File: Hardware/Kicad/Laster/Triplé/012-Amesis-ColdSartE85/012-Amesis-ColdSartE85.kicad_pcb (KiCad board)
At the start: 2 copper layers, 52.1 x 54.9 mm, 24 parts, among them J1 Screw_Terminal_01x02, J2 Conn_01x05_Female, J3 Conn_01x03_Female

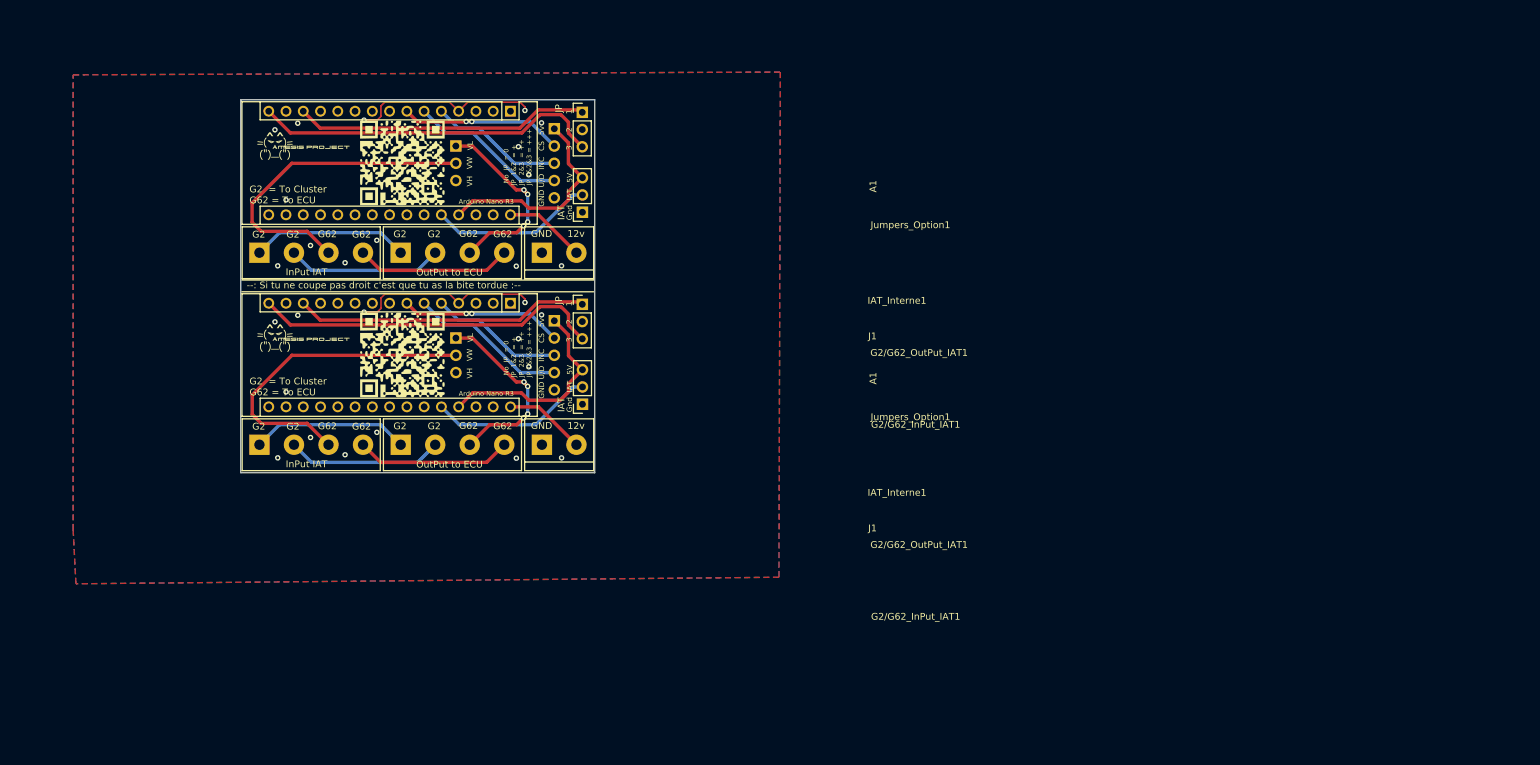
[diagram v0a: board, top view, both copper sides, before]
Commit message: maj
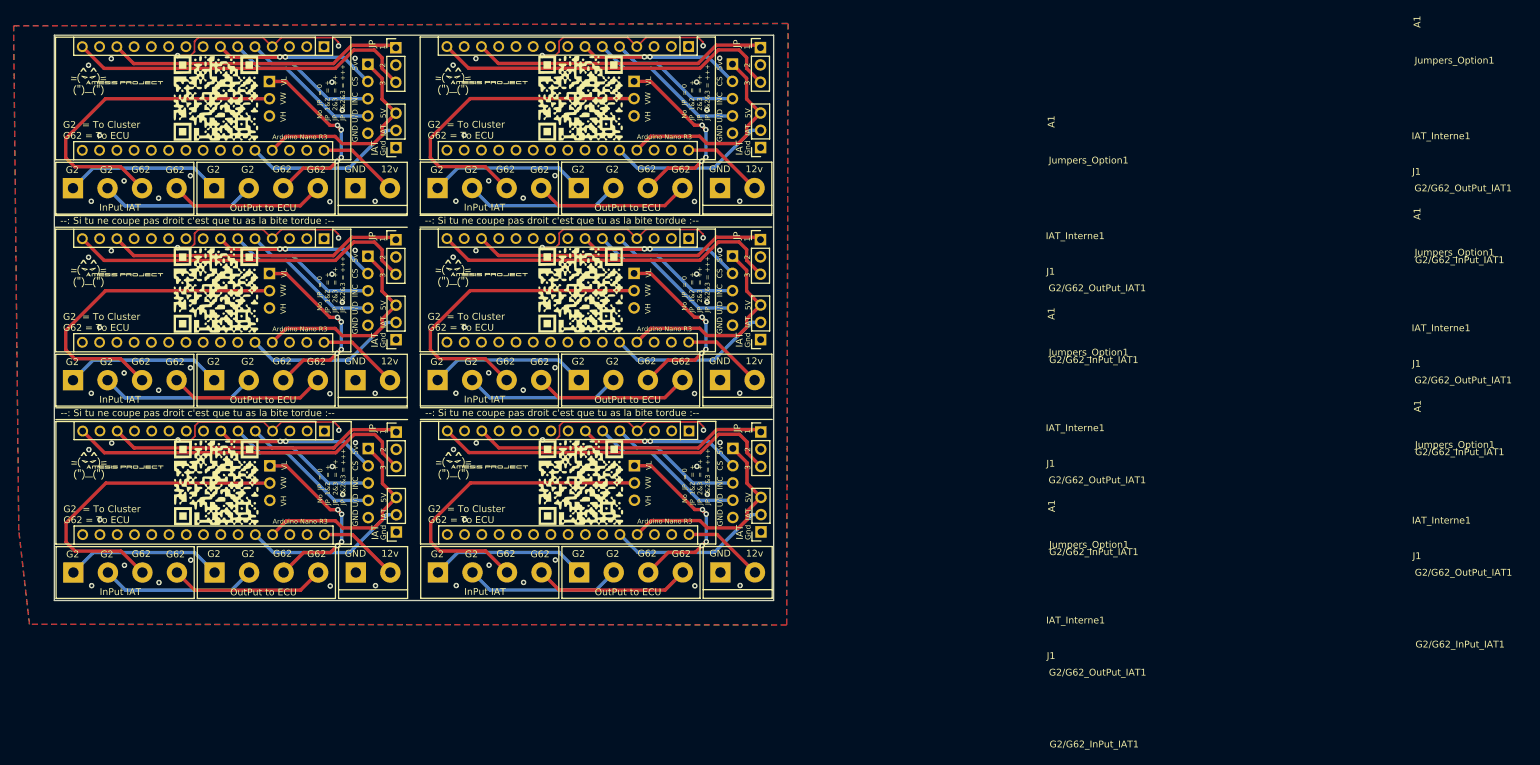
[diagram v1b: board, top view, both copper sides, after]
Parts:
- added  : LOGO, AP_Amesis Logo:AmesisProject Logo 15mm, F.Cu at (99.0, 51.5)
- added  : LOGO, AP_Amesis Logo:AmesisProject Logo 15mm, F.Cu at (99.1, 79.8)
- added  : LOGO, AP_Amesis Logo:AmesisProject Logo 30mm, B.Cu at (105.5, 51.7)
- added  : LOGO, AP_Amesis Logo:10x10 KiCad QR Code La Boutique Amesis Project, B.Cu at (128.8, 24.2)
- added  : LOGO, AP_Amesis Logo:AmesisProject Logo 30mm, B.Cu at (105.5, 80.0)
- added  : LOGO, AP_Amesis Logo:AmesisProject Logo 30mm, B.Cu at (105.5, 23.5)
- added  : LOGO, AP_Amesis Logo:10x10 KiCad QR Code La Boutique Amesis Project, B.Cu at (182.5, 80.7)
- added  : LOGO, AP_Amesis Logo:10x10 KiCad QR Code La Boutique Amesis Project, B.Cu at (128.9, 80.8)
- added  : LOGO, AP_Amesis Logo:15x15 KiCad QR Code La Boutique Amesis Project, F.Cu at (167.4, 81.5)
- added  : LOGO, AP_Amesis Logo:10x10 KiCad QR Code La Boutique Amesis Project, B.Cu at (128.8, 52.5)
- added  : LOGO, AP_Amesis Logo:AmesisProject Logo 30mm, B.Cu at (159.2, 80.0)
- added  : LOGO, AP_Amesis Logo:15x15 KiCad QR Code La Boutique Amesis Project, F.Cu at (113.8, 81.5)
- added  : LOGO, AP_Amesis Logo:15x15 KiCad QR Code La Boutique Amesis Project, F.Cu at (113.7, 24.9)
- added  : LOGO, AP_Amesis Logo:AmesisProject Logo 15mm, F.Cu at (99.0, 23.3)
- added  : LOGO, AP_Amesis Logo:AmesisProject Logo 15mm, F.Cu at (152.7, 79.8)
- added  : LOGO, AP_Amesis Logo:15x15 KiCad QR Code La Boutique Amesis Project, F.Cu at (113.7, 53.2)
- added A1: Arduino_Nano_v3.x, Module:Arduino_Nano, F.Cu at (129.6, 45.8)
- added A1: Arduino_Nano_v3.x, Module:Arduino_Nano, F.Cu at (183.3, 74.1)
- added A1: Arduino_Nano_v3.x, Module:Arduino_Nano, F.Cu at (129.7, 74.1)
- added A1: Arduino_Nano_v3.x, Module:Arduino_Nano, F.Cu at (129.6, 17.6)
- added G2/G62_InPut_IAT1: Conn_01x04_Male, TerminalBlock:TerminalBlock_bornier-4_P5.08mm, F.Cu at (146.4, 94.9)
- added G2/G62_InPut_IAT1: Conn_01x04_Male, TerminalBlock:TerminalBlock_bornier-4_P5.08mm, F.Cu at (92.7, 38.4)
- added G2/G62_InPut_IAT1: Conn_01x04_Male, TerminalBlock:TerminalBlock_bornier-4_P5.08mm, F.Cu at (92.8, 95.0)
- added G2/G62_InPut_IAT1: Conn_01x04_Male, TerminalBlock:TerminalBlock_bornier-4_P5.08mm, F.Cu at (92.7, 66.7)
- added G2/G62_OutPut_IAT1: Conn_01x04_Male, TerminalBlock:TerminalBlock_bornier-4_P5.08mm, F.Cu at (113.5, 66.7)
- added G2/G62_OutPut_IAT1: Conn_01x04_Male, TerminalBlock:TerminalBlock_bornier-4_P5.08mm, F.Cu at (113.5, 38.4)
- added G2/G62_OutPut_IAT1: Conn_01x04_Male, TerminalBlock:TerminalBlock_bornier-4_P5.08mm, F.Cu at (167.2, 94.9)
- added G2/G62_OutPut_IAT1: Conn_01x04_Male, TerminalBlock:TerminalBlock_bornier-4_P5.08mm, F.Cu at (113.5, 95.0)
- added IAT_Interne1: R_Potentiometer, Connector_PinSocket_2.54mm:PinSocket_1x03_P2.54mm_Vertical, F.Cu at (140.2, 60.7)
- added IAT_Interne1: R_Potentiometer, Connector_PinSocket_2.54mm:PinSocket_1x03_P2.54mm_Vertical, F.Cu at (193.9, 89.0)
- added IAT_Interne1: R_Potentiometer, Connector_PinSocket_2.54mm:PinSocket_1x03_P2.54mm_Vertical, F.Cu at (140.2, 32.4)
- added IAT_Interne1: R_Potentiometer, Connector_PinSocket_2.54mm:PinSocket_1x03_P2.54mm_Vertical, F.Cu at (140.3, 89.0)
- added J1: Screw_Terminal_01x02, TerminalBlock:TerminalBlock_bornier-2_P5.08mm, F.Cu at (188.0, 94.9)
- added J1: Screw_Terminal_01x02, TerminalBlock:TerminalBlock_bornier-2_P5.08mm, F.Cu at (134.3, 66.7)
- added J1: Screw_Terminal_01x02, TerminalBlock:TerminalBlock_bornier-2_P5.08mm, F.Cu at (134.3, 95.0)
- added J1: Screw_Terminal_01x02, TerminalBlock:TerminalBlock_bornier-2_P5.08mm, F.Cu at (134.3, 38.4)
- added J2: Conn_01x05_Female, Connector_PinSocket_2.54mm:PinSocket_1x05_P2.54mm_Vertical, B.Cu at (136.1, 48.4)
- added J2: Conn_01x05_Female, Connector_PinSocket_2.54mm:PinSocket_1x05_P2.54mm_Vertical, B.Cu at (136.1, 76.7)
- added J2: Conn_01x05_Female, Connector_PinSocket_2.54mm:PinSocket_1x05_P2.54mm_Vertical, B.Cu at (189.8, 76.7)
- added J2: Conn_01x05_Female, Connector_PinSocket_2.54mm:PinSocket_1x05_P2.54mm_Vertical, B.Cu at (136.1, 20.2)
- added J3: Conn_01x03_Female, Connector_PinSocket_2.54mm:PinSocket_1x03_P2.54mm_Vertical, B.Cu at (121.6, 51.0)
- added J3: Conn_01x03_Female, Connector_PinSocket_2.54mm:PinSocket_1x03_P2.54mm_Vertical, B.Cu at (175.3, 79.2)
- added J3: Conn_01x03_Female, Connector_PinSocket_2.54mm:PinSocket_1x03_P2.54mm_Vertical, B.Cu at (121.7, 79.3)
- added J3: Conn_01x03_Female, Connector_PinSocket_2.54mm:PinSocket_1x03_P2.54mm_Vertical, B.Cu at (121.6, 22.7)
- added Jumpers_Option1: Conn_01x03_Male, Connector_PinHeader_2.54mm:PinHeader_1x03_P2.54mm_Vertical, F.Cu at (193.9, 74.3)
- added Jumpers_Option1: Conn_01x03_Male, Connector_PinHeader_2.54mm:PinHeader_1x03_P2.54mm_Vertical, F.Cu at (140.2, 17.7)
- added Jumpers_Option1: Conn_01x03_Male, Connector_PinHeader_2.54mm:PinHeader_1x03_P2.54mm_Vertical, F.Cu at (140.2, 46.0)
- added Jumpers_Option1: Conn_01x03_Male, Connector_PinHeader_2.54mm:PinHeader_1x03_P2.54mm_Vertical, F.Cu at (140.3, 74.3)
- moved   27.9 mm to (182.5, 52.4)
- moved   27.9 mm to (182.5, 24.2)
- moved   27.9 mm to (159.1, 51.7)
- moved G2/G62_InPut_IAT1 27.9 mm to (146.4, 66.6)
- moved G2/G62_OutPut_IAT1 27.9 mm to (167.1, 66.6)
- moved G2/G62_OutPut_IAT1 27.9 mm to (167.1, 38.4)
- moved IAT_Interne1 27.9 mm to (193.9, 60.7)
- moved IAT_Interne1 27.9 mm to (193.9, 32.4)
- moved J1 27.9 mm to (187.9, 38.4)
- moved J2 27.9 mm to (189.7, 20.1)
- moved Jumpers_Option1 27.9 mm to (193.8, 17.7)
- moved Jumpers_Option1 27.9 mm to (193.9, 46.0)
- moved   27.9 mm to (152.7, 51.5)
- moved   27.9 mm to (152.6, 23.2)
- moved   27.9 mm to (167.4, 24.9)
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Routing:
- net Net-(A1-Pad15): track 102.9 -> 308.7 mm
- net Net-(G2/G62_InPut_IAT1-Pad3): track 96.6 -> 289.9 mm
- net Net-(A1-Pad13): track 86.7 -> 260.1 mm
- net Net-(A1-Pad27): track 62.0 -> 185.9 mm
- net Net-(G2/G62_OutPut_IAT1-Pad3): track 59.7 -> 179.0 mm, vias 8 -> 24
- net GND: track 55.1 -> 165.4 mm, vias 28 -> 84
- net Net-(A1-Pad7): track 49.3 -> 148.0 mm, vias 4 -> 12
- net Net-(A1-Pad26): track 48.3 -> 144.8 mm
- net Net-(A1-Pad6): track 46.8 -> 140.3 mm
- net Net-(G2/G62_InPut_IAT1-Pad1): track 46.4 -> 139.3 mm
- net Net-(G2/G62_InPut_IAT1-Pad4): track 45.8 -> 137.5 mm
- net Net-(G2/G62_InPut_IAT1-Pad2): track 45.8 -> 137.5 mm
- net Net-(A1-Pad5): track 39.6 -> 118.7 mm
- net Net-(A1-Pad30): track 24.0 -> 72.1 mm
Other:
- board size 52.1 x 54.9 mm -> 105.8 x 83.2 mm
